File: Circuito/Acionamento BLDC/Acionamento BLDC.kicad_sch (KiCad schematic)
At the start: 40 parts, among them J1 42V, J2 Motor, J3 Hall, J4 Potenciômetro, Q1 FDH50N50, Q2 FDH50N50, Q3 FDH50N50, Q4 FDH50N50, Q5 FDH50N50, Q6 FDH50N50, U1 MC33035

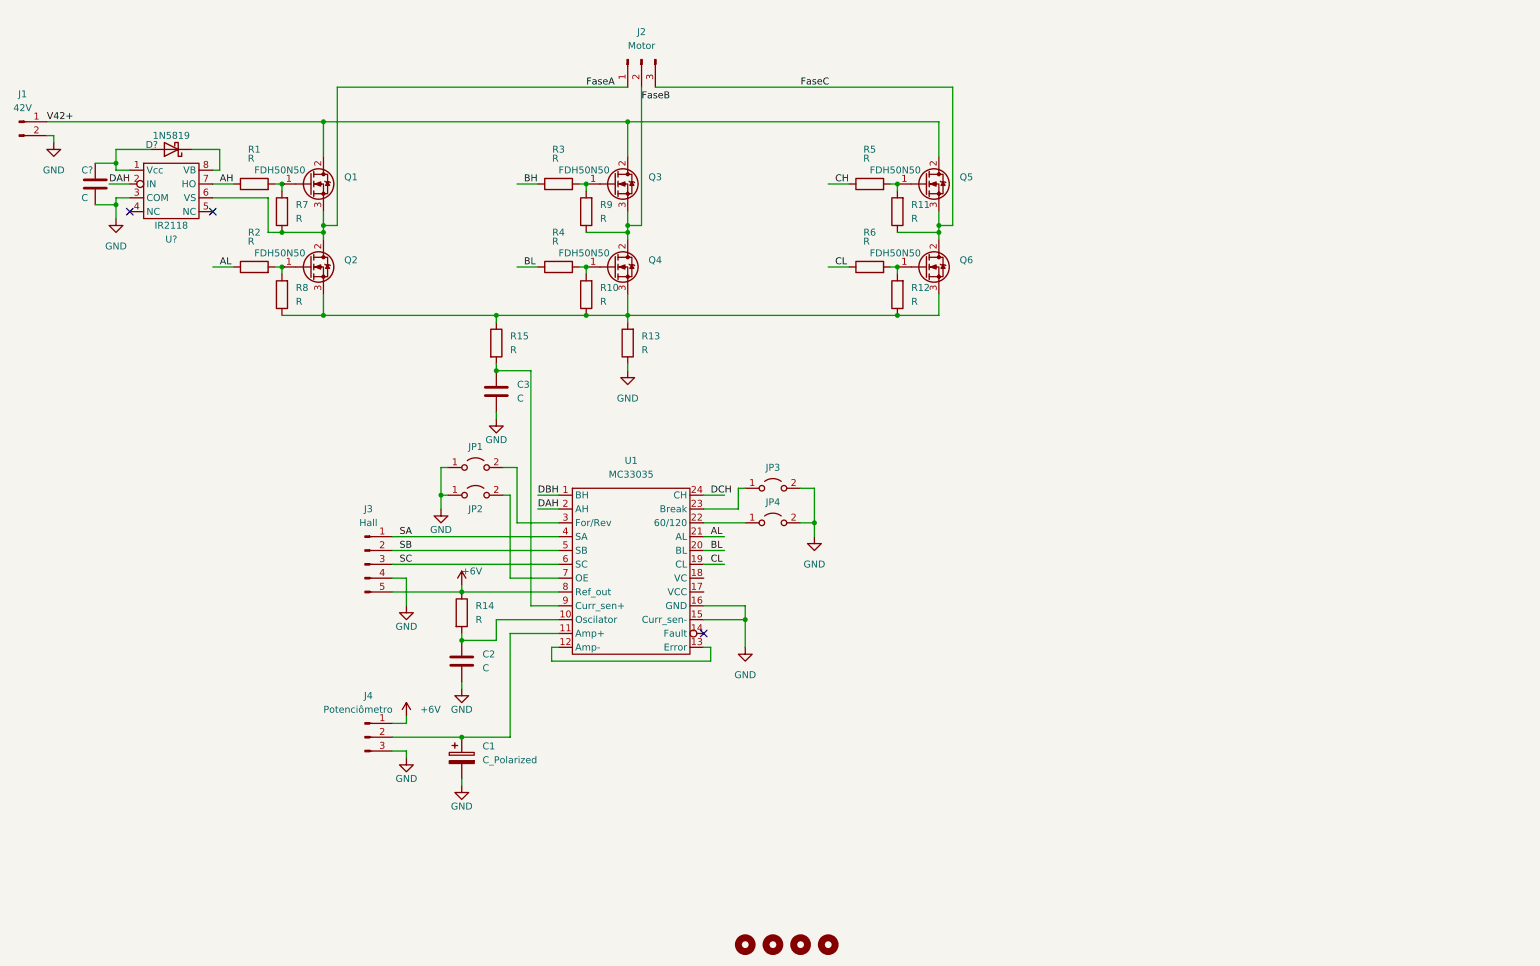
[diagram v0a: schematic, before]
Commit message: Versão 2023
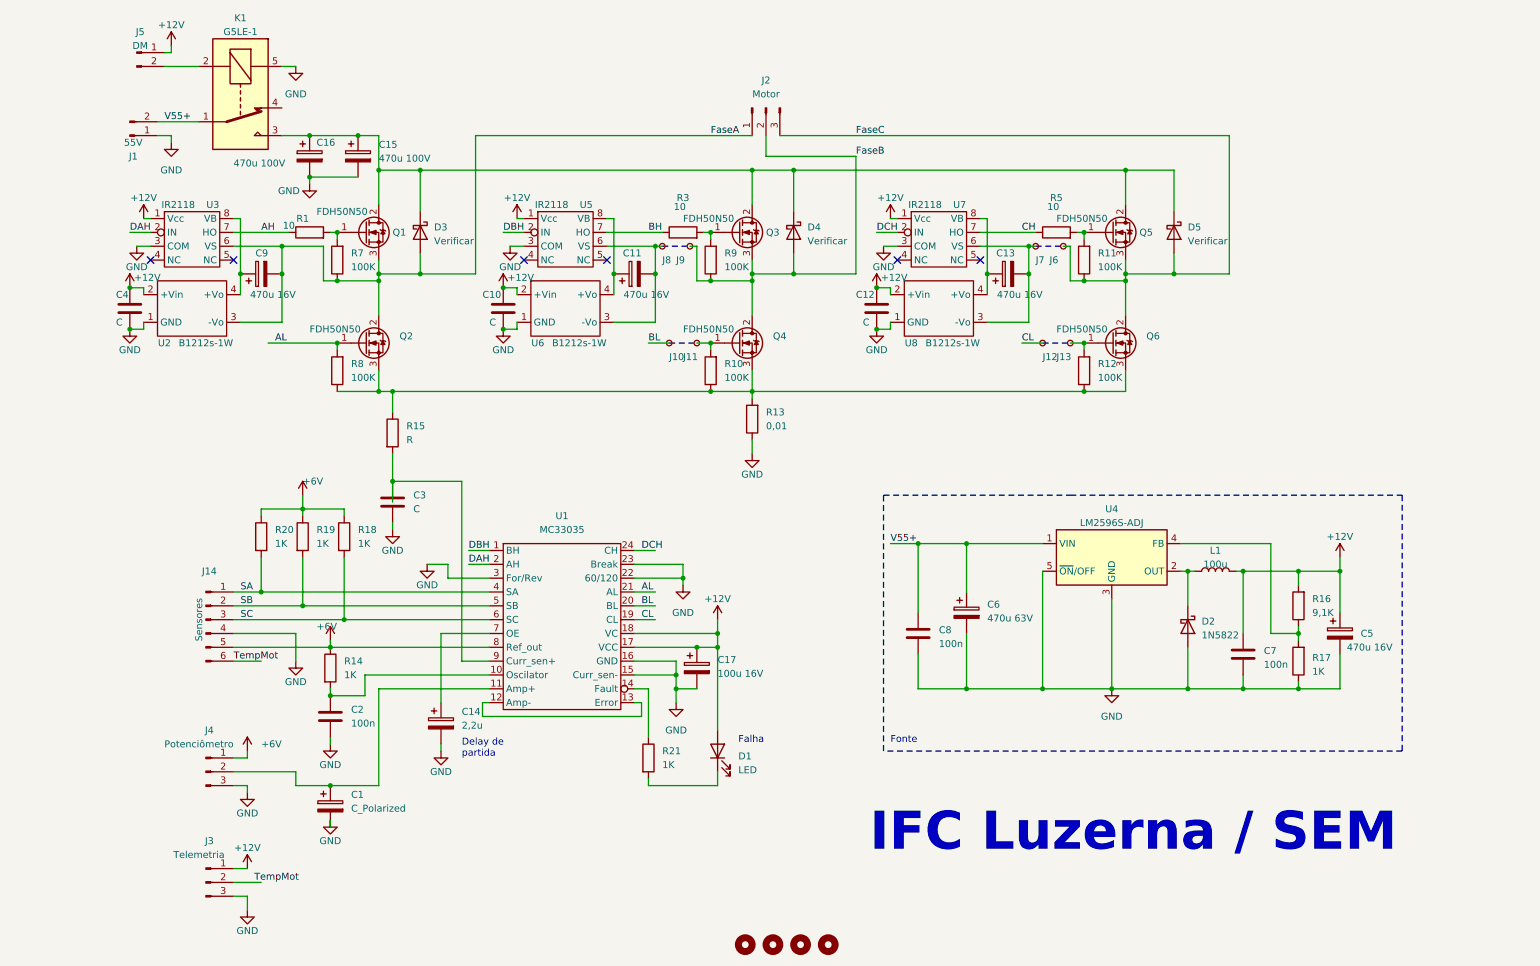
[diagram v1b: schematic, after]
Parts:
- removed D?: 1N5819, Diode_THT:D_DO-41_SOD81_P10.16mm_Horizontal, symbol Diode:1N5819
- removed J3: Hall, Connector_Phoenix_MC:PhoenixContact_MC_1,5_5-G-3.81_1x05_P3.81mm_Horizontal, symbol Connector:Conn_01x05_Male
- removed JP1, JP2, JP3, JP4: Jumper_2_Open, Connector_PinHeader_2.54mm:PinHeader_1x02_P2.54mm_Vertical, symbol Jumper:Jumper_2_Open
- removed R2, R4, R6: R, Resistor_THT:R_Axial_DIN0207_L6.3mm_D2.5mm_P10.16mm_Horizontal, symbol Device:R
- added C10, C12: C, Capacitor_THT:C_Disc_D9.0mm_W2.5mm_P5.00mm, symbol Device:C
- added C11, C13, C5, C9: 470u 16V, Capacitor_THT:CP_Radial_D10.0mm_P3.50mm, symbol Device:C_Polarized
- added C14: 2,2u, Capacitor_THT:CP_Radial_D4.0mm_P2.00mm, symbol Device:C_Polarized
- added C15, C16: 470u 100V, Capacitor_THT:CP_Radial_D22.0mm_P10.00mm_SnapIn, symbol Device:C_Polarized
- added C17: 100u 16V, Capacitor_THT:CP_Radial_D8.0mm_P2.50mm, symbol Device:C_Polarized
- added C6: 470u 63V, Capacitor_THT:CP_Radial_D13.0mm_P5.00mm, symbol Device:C_Polarized
- added C7, C8: 100n, Capacitor_THT:C_Axial_L5.1mm_D3.1mm_P7.50mm_Horizontal, symbol Device:C
- added D1: LED, LED_THT:LED_D5.0mm, symbol Device:LED
- added D2: 1N5822, Diode_THT:D_DO-201AD_P15.24mm_Horizontal, symbol Diode:1N5822
- added D3, D4, D5: Verificar, Package_TO_SOT_THT:TO-220-2_Vertical, symbol Diode:1N5822
- added J10, J11, J12, J13, J6, J7, J8, J9: ~, TestPoint:TestPoint_Loop_D3.50mm_Drill0.9mm_Beaded, symbol Connector:TestPoint_Small
- added J14: Sensores, Connector_Phoenix_MC:PhoenixContact_MC_1,5_6-G-3.81_1x06_P3.81mm_Horizontal, symbol Connector:Conn_01x06_Pin
- added J3: Telemetria, Connector_Phoenix_MC:PhoenixContact_MC_1,5_3-G-3.81_1x03_P3.81mm_Horizontal, symbol Connector:Conn_01x03_Male
- added J5: DM, Connector_Phoenix_MC:PhoenixContact_MC_1,5_2-G-3.81_1x02_P3.81mm_Horizontal, symbol Connector:Conn_01x02_Male
- added K1: G5LE-1, Relay_THT:Relay_SPDT_Omron-G5LE-1, symbol Relay:G5LE-1
- added L1: 100u, Inductor_SMD:L_12x12mm_H6mm, symbol Device:L
- added R16: 9,1K, Resistor_THT:R_Axial_DIN0207_L6.3mm_D2.5mm_P10.16mm_Horizontal, symbol Device:R
- added R17, R18, R19, R20, R21: 1K, Resistor_THT:R_Axial_DIN0207_L6.3mm_D2.5mm_P10.16mm_Horizontal, symbol Device:R
- added U2, U6, U8: B1212s-1W, B1212s-1W:B1212s-1W, symbol MC33035:B1212s-1W
- added U4: LM2596S-ADJ, Package_TO_SOT_SMD:TO-263-5_TabPin3, symbol Regulator_Switching:LM2596S-ADJ
- added U5, U7: IR2118, Package_DIP:DIP-8_W7.62mm_LongPads, symbol MC33035:IR2118
- C2: value C -> 100n
- J1: value 42V -> 55V
- R1, R3, R5: value R -> 10
- R10, R11, R12, R7, R8, R9: value R -> 100K
- R13: value R -> 0,01; footprint Resistor_THT:R_Axial_DIN0207_L6.3mm_D2.5mm_P10.16mm_Horizontal -> Resistor_THT:R_Axial_Power_L25.0mm_W9.0mm_P27.94mm
- R14: value R -> 1K
- U3: renamed from U?; footprint (none) -> Package_DIP:DIP-8_W7.62mm_LongPads
- gave numbers to parts that had none: 1
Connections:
- net +6V: now also J14.5 (Pin_5), R18.1, R19.1, R20.1
- net AL: now also Q2.1 (G), R8.2
- net BH: now also U5.7 (HO)
- net BL: now also J10.1
- net CH: now also U7.7 (HO)
- net CL: now also J12.1
- net DBH: now also U5.2 (IN)
- net DCH: now also U7.2 (IN)
- net FaseA: now also C9.2, D3.2 (A), U2.3 (-Vo)
- net FaseB: now also D4.2 (A), J9.1
- net FaseC: now also D5.2 (A), J6.1
- net GND: now also J1.1 (Pin_1), U1.22 (60/120), U1.23 (Break), U1.3 (For/Rev), C10.2, C12.2, C14.2, C15.2, C16.2, C17.2, C5.2, C6.2, C7.2, C8.2, D2.2 (A), J14.4 (Pin_4), J3.3 (Pin_3), K1.5, R17.1, U2.1 (GND), U4.3 (GND), U4.5 (~{ON}/OFF), U5.3 (COM), U6.1 (GND), U7.3 (COM), U8.1 (GND); no longer J1.2 (Pin_2)
- net SA: now also J14.1 (Pin_1), R20.2
- net SB: now also J14.2 (Pin_2), R19.2
- net SC: now also J14.3 (Pin_3), R18.2
- net at U1.14 (Fault): now also R21.1
- net +12V: now reaches U1.17 (VCC)
- net +12V: now also C4.1, U1.18 (VC), U3.1 (Vcc), C10.1, C12.1, C17.1, C5.1, C7.1, D1.2 (A), J3.1 (Pin_1), J5.1 (Pin_1), L1.2, R16.2, U2.2 (+Vin), U5.1 (Vcc), U6.2 (+Vin), U7.1 (Vcc), U8.2 (+Vin)
- net at U1.7 (OE): now also C14.1
- net at Q6.1 (G), R12.2: now also J13.1
- net at U3.8 (VB): now also C9.1, U2.4 (+Vo)
- net at Q4.1 (G), R10.2: now also J11.1
- net V42+: no longer names the net of Q1.2 (D), Q3.2 (D), Q5.2 (D)
- net V42+: now also C15.1, C16.1, D3.1 (K), D4.1 (K), D5.1 (K), K1.3; no longer J1.1 (Pin_1)
- new net: J5.2 (Pin_2), K1.2
- new net: C13.2, J7.1, U7.6 (VS), U8.3 (-Vo)
- new net: C13.1, U7.8 (VB), U8.4 (+Vo)
- new net: D2.1 (K), L1.1, U4.2 (OUT)
- new net: R16.1, R17.2, U4.4 (FB)
- new net: C11.1, U5.8 (VB), U6.4 (+Vo)
- new net: C11.2, J8.1, U5.6 (VS), U6.3 (-Vo)
- new net: D1.1 (K), R21.2
- new net TempMot: J14.6 (Pin_6), J3.2 (Pin_2)
- new net V55+: C6.1, C8.1, J1.2 (Pin_2), K1.1, U4.1 (VIN)
- no-connect marks 3 -> 6
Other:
- note added: "Delay de partida"
- note added: "Falha"
- note added: "Fonte"
- note added: "IFC Luzerna / SEM"
- title: (none) -> Acionamento BLDC Símples
- moved on the sheet: C1, C2, C3, C4, J1, J2, J4, Q1, Q2, Q3, Q4, Q5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
